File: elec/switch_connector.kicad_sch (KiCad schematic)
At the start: 8 parts, among them J3 BM04B-SRSS-TB, Q1 2N7002

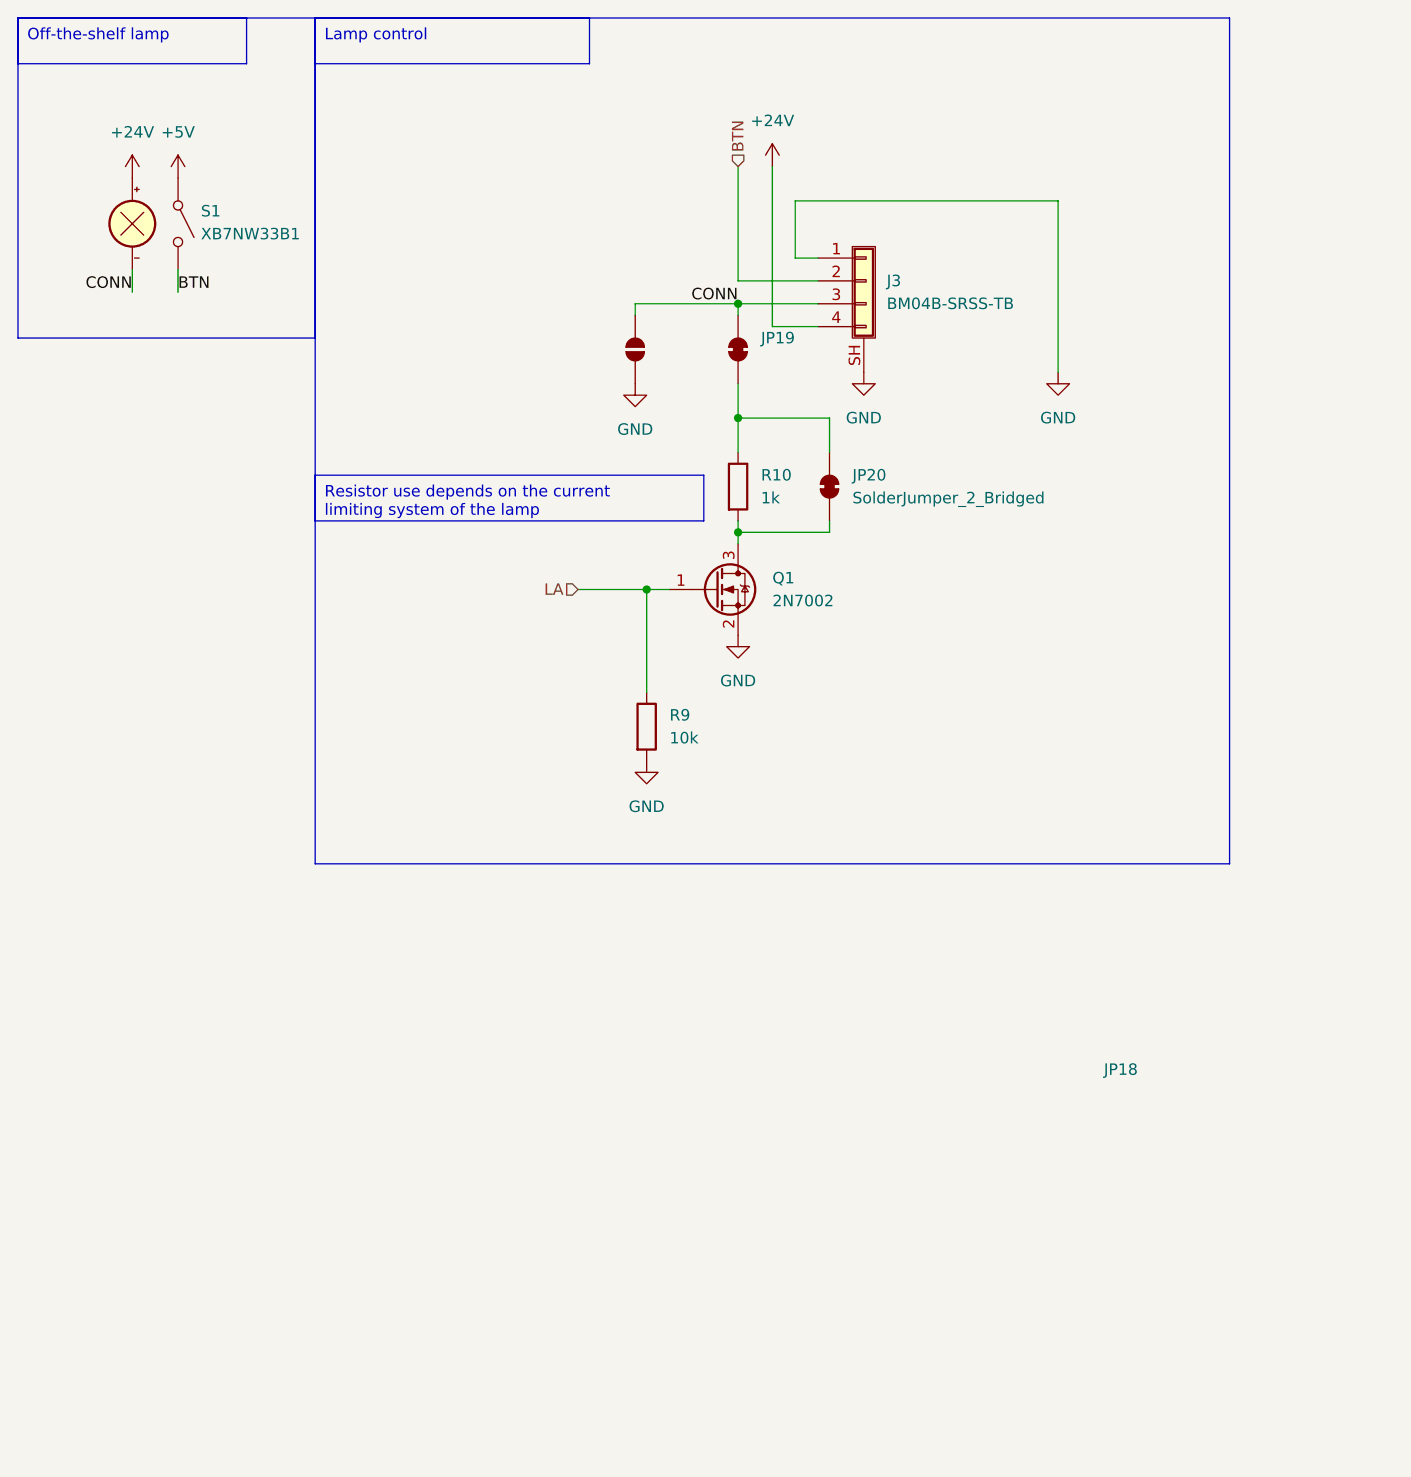
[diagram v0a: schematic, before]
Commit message: v1 3D print PCB
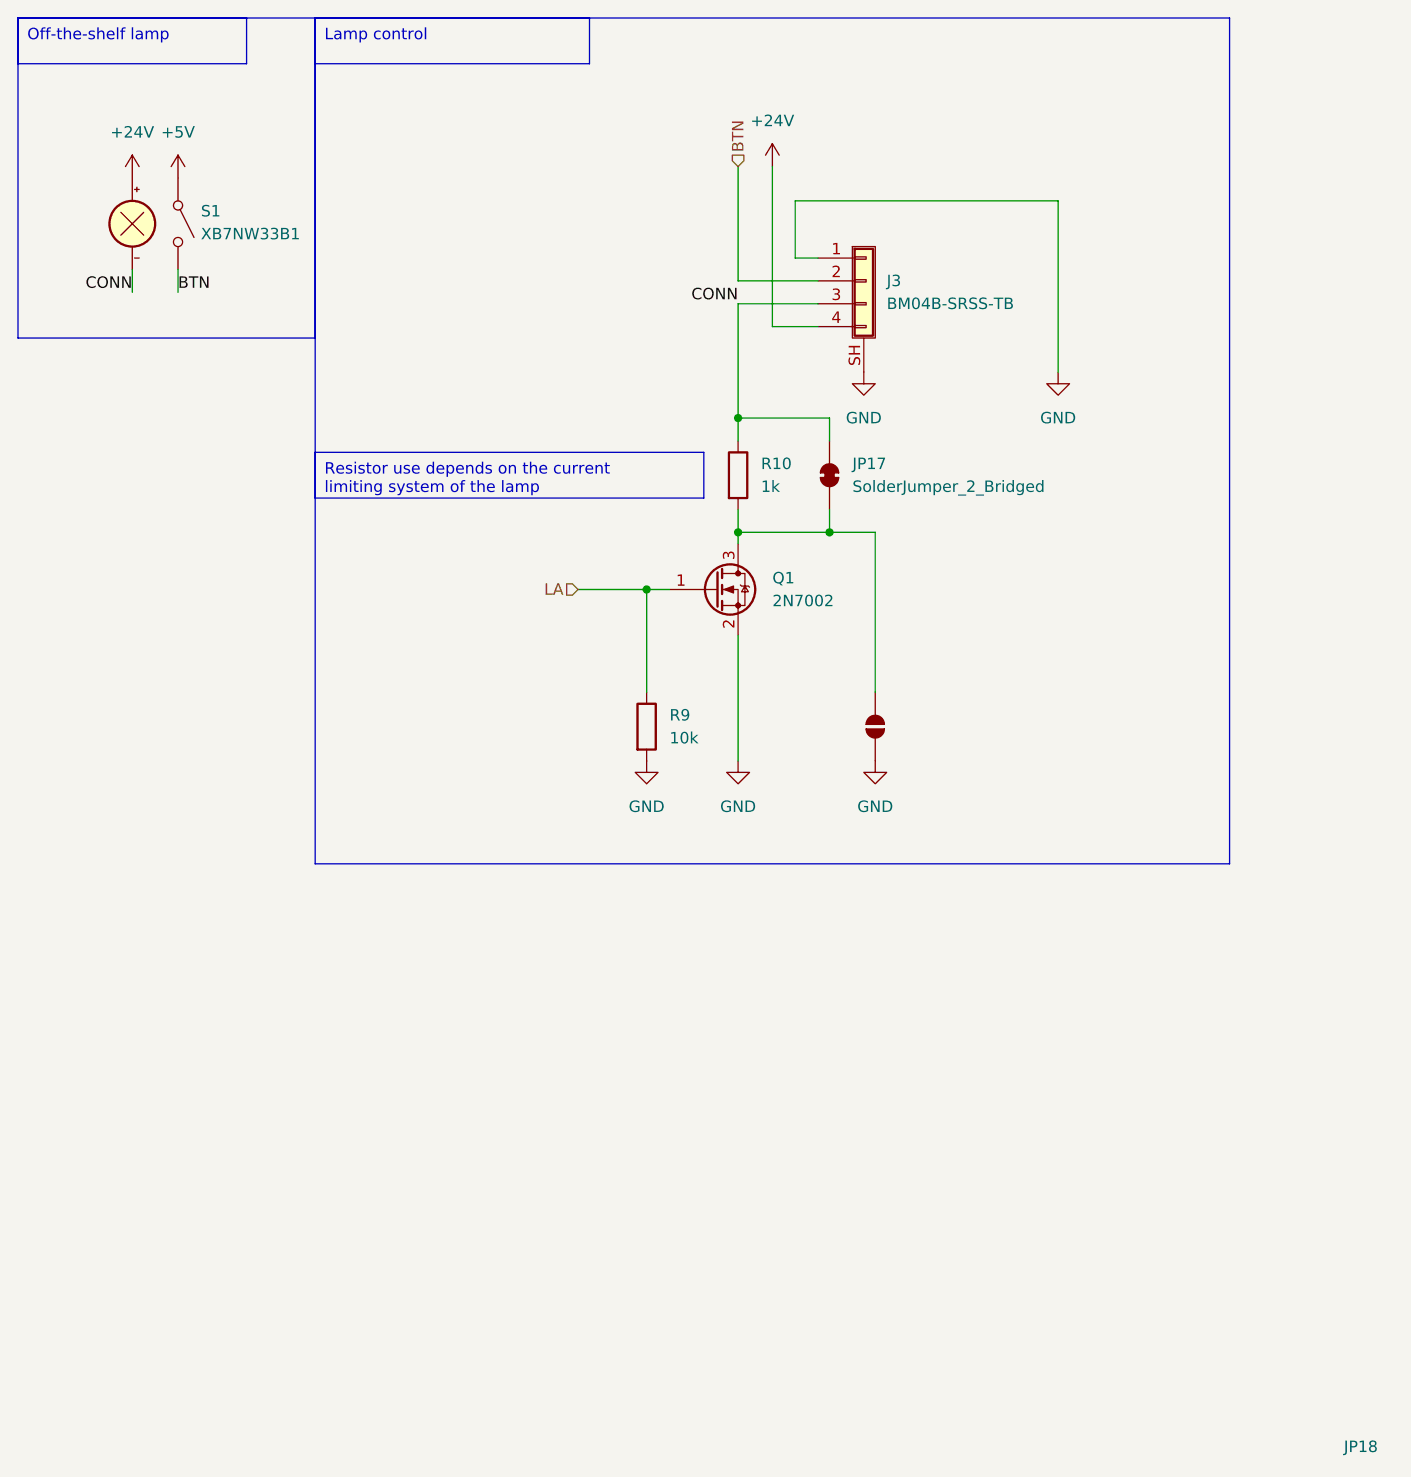
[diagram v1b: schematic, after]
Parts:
- removed JP19: SolderJumper_2_Bridged, Jumper:SolderJumper-2_P1.3mm_Bridged_Pad1.0x1.5mm, symbol Jumper:SolderJumper_2_Bridged
- renumbered JP20 to JP17
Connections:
- net CONN: now also JP17.2 (B), R10.1; no longer JP18.1 (A)
- net at JP17.1 (A), Q1.3 (D), R10.2: now also JP18.1 (A)
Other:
- moved on the sheet: JP17, JP18, R10
